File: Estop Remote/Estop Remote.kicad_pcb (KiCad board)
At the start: 2 copper layers, 64.8 x 26.7 mm, 5 parts, among them J1 Enable Out, J2 Power, U1 AdafruitFeatherM0LoRa

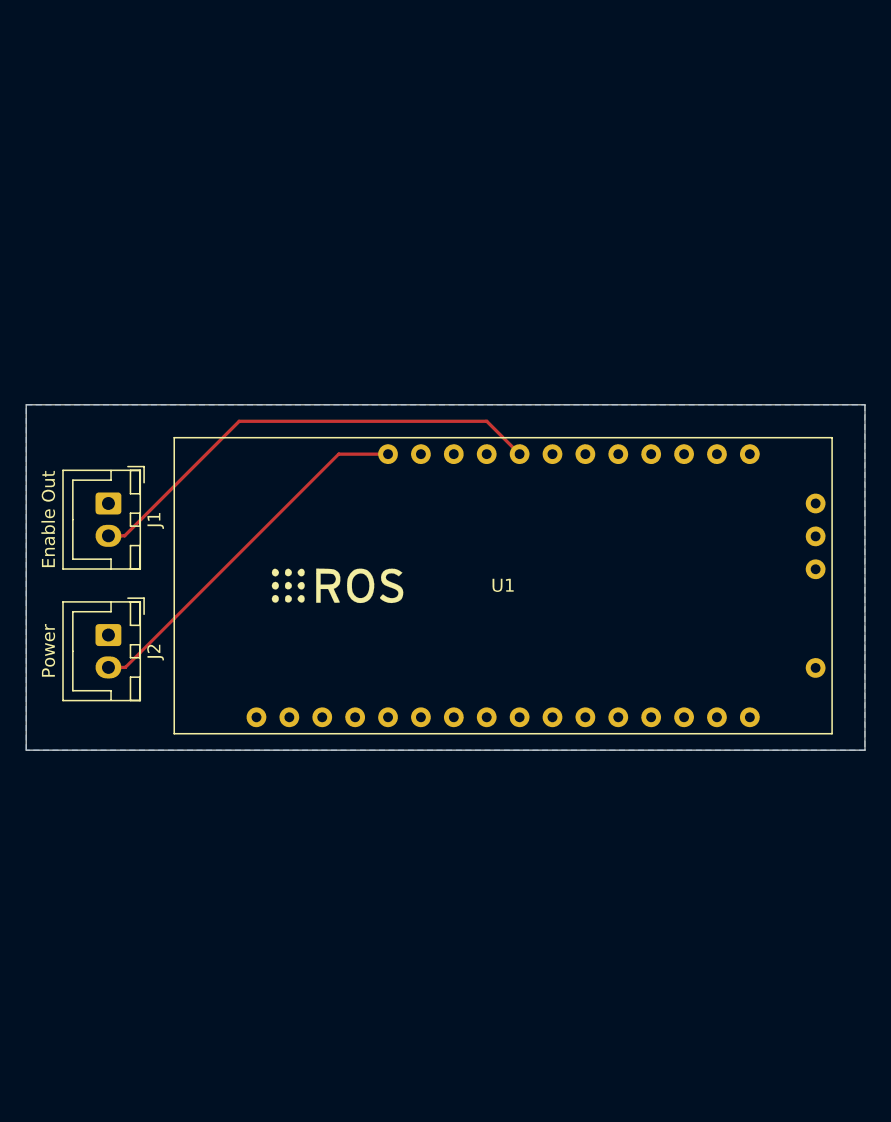
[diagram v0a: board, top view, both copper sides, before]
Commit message: Estop Remote First Draft
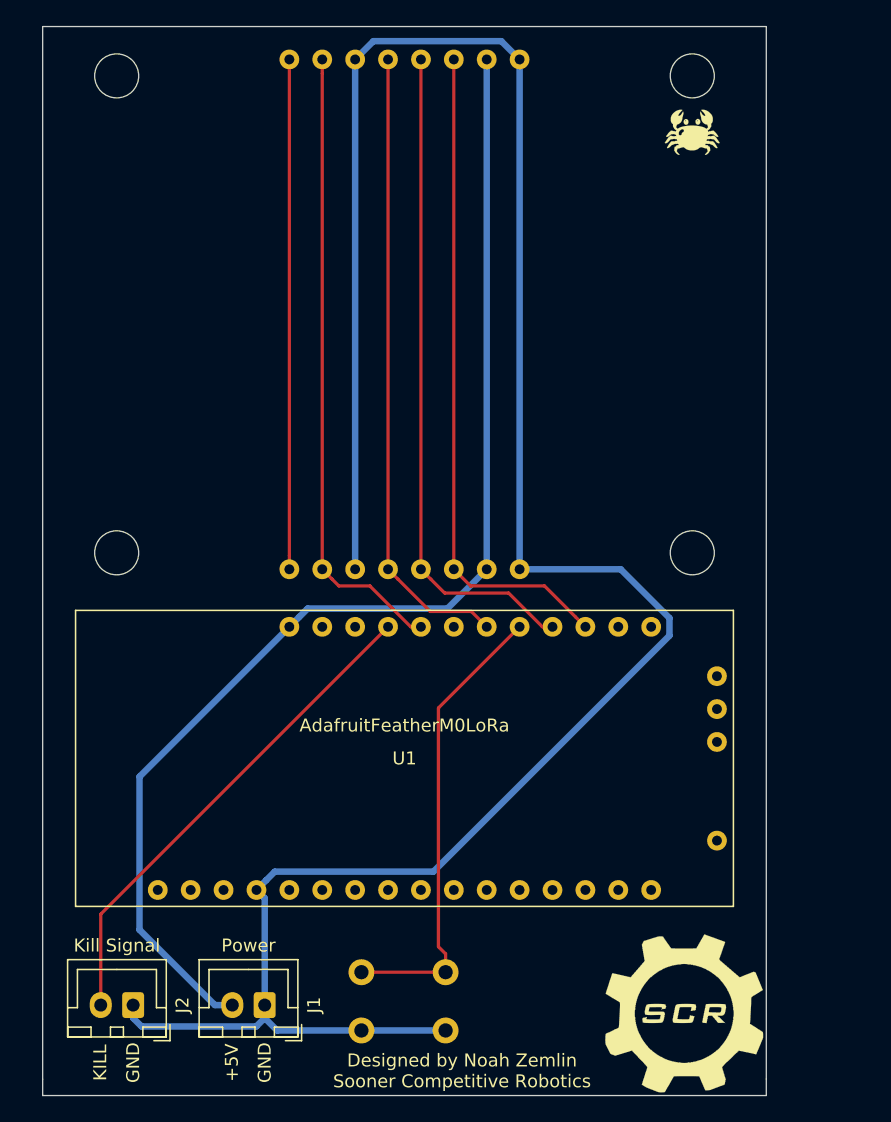
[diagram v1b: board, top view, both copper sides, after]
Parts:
- removed the G*** at (144.8, 82.5)
- removed the G*** at (170.2, 82.5)
- added G***: LOGO, SCR_KiCAD_Lib:crab-image, F.Cu at (172.1, 47.6)
- added G***: LOGO, SCR_KiCAD_Lib:scr-logo, B.Cu at (171.4, 115.6)
- added G***: LOGO, SCR_KiCAD_Lib:scr-logo, F.Cu at (171.4, 115.6)
- added SW1: Stop Button, Button_Switch_THT:SW_PUSH_6mm_H5mm, B.Cu at (153.0, 112.4)
- added U2: Nokia5110LED, SCR_KiCAD_Lib:AdafruitNokia5110, B.Cu at (149.9, 63.5)
- J1: value Enable Out -> Power
- J2: value Power -> Kill Signal
- moved J1 40.6 mm to (139.1, 114.9), turned to 180 degrees
- moved J2 28.6 mm to (128.9, 114.9), turned to 180 degrees
- moved U1 15.4 mm to (124.5, 107.3)
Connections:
- J1 pad 2: Net-(J1-Pad2) -> +5V
- J2 pad 2: VCC -> SIG_KILL
- U1 pad 10: Net-(U1-Pad10) -> DSPL_DC
- U1 pad 12: Net-(J1-Pad2) -> DSPL_RST
- U1 pad 13: Net-(U1-Pad13) -> SIG_KILL
- U1 pad 16: VCC -> +5V
- U1 pad 7: Net-(U1-Pad7) -> DSPL_SCLK
- U1 pad 8: Net-(U1-Pad8) -> DSPL_DIN
- U1 pad 9: Net-(U1-Pad9) -> SIG_STOP
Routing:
- net GND: track 0.00 -> 183.6 mm
- net +5V: track 0.00 -> 94.2 mm
- net DSPL_SCLK: track 0.00 -> 51.4 mm
- net DSPL_DIN: track 0.00 -> 51.4 mm
- net DSPL_DC: track 0.00 -> 48.8 mm
- net DSPL_RST: track 0.00 -> 48.8 mm
- net Net-(U2-Pad8): track 0.00 -> 39.4 mm
- net SIG_KILL: track 0.00 -> 38.4 mm
- net Net-(J1-Pad2): track 36.5 -> 0.00 mm
- net SIG_STOP: track 0.00 -> 36.0 mm
- net VCC: track 28.4 -> 0.00 mm
- removed copper zone on B.Cu, net GND
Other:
- board size 64.8 x 26.7 mm -> 55.9 x 82.6 mm
- net class Default: clearance 0.2 -> 0.3
- net class POWER added: clearance 0.4, trace_width 0.5, via_dia 0.8, via_drill 0.4
- rule pad_to_mask_clearance: 0.051 -> 0
- rule trace_clearance: 0.2 -> 0.3
- board text added: "+5V"
- board text added: "Designed by Noah Zemlin Sooner Competitive Robotics"
- board text added: "GND"
- board text added: "KILL"
